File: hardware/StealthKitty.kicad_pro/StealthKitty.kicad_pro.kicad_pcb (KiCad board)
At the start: 4 copper layers, 53.9 x 57 mm, 82 parts, among them IC501 MP1475DJ-LF-P, J201 Conn_01x06, J202 Conn_01x06, J301 Conn_01x06, J302 Conn_01x06, J303 Conn_01x08, J401 Conn_ST_STDC14, SW401 SW_Push, SW402 SW_Push, SW501 Switch, U1 ZXBM5210-SP, U2 ZXBM5210-SP, U301 ADXL343, U401 STM32G431CBU6, Y401 Crystal_GND24_Small

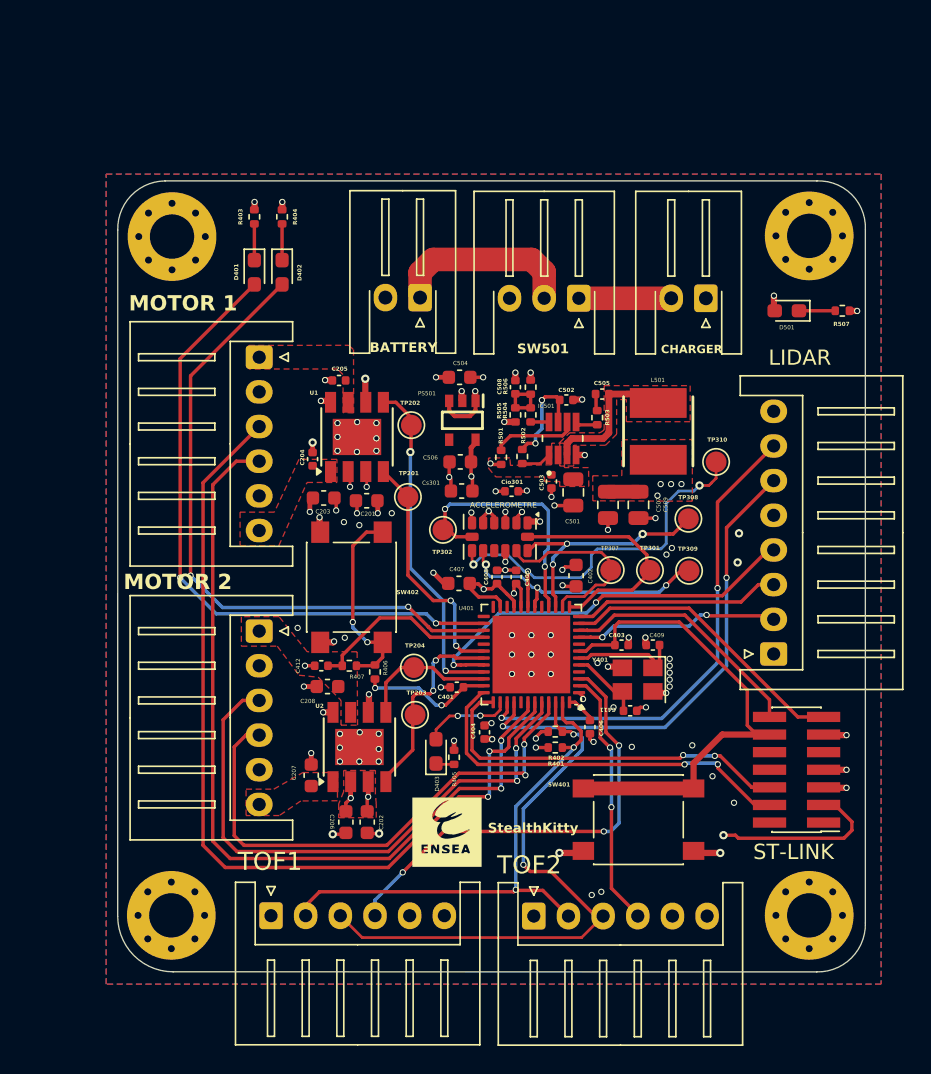
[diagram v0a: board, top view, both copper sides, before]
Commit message: Ajout fichier GERBER zip
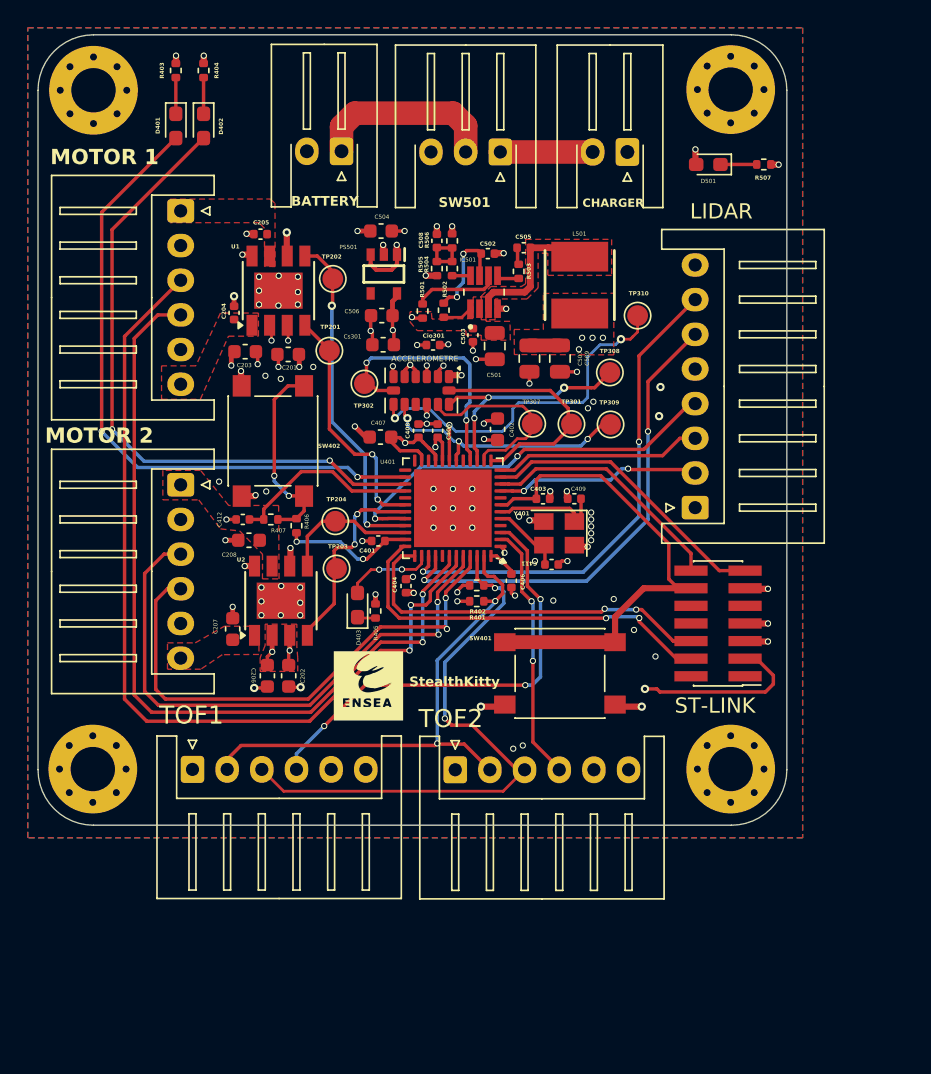
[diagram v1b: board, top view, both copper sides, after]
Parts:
- moved C206 12.0 mm to (135.1, 102.2)
- moved C509 12.0 mm to (154.6, 79.3)
- moved Cs301 12.0 mm to (141.9, 78.3)
- moved J302 12.0 mm to (128.1, 109.0)
- moved J303 12.0 mm to (164.4, 90.1)
- moved R401 12.0 mm to (148.6, 96.8)
- moved BT501 12.0 mm to (138.9, 64.4)
- moved C204 12.0 mm to (131.1, 76.0)
- moved C402 12.0 mm to (150.1, 84.5)
- moved C406 12.0 mm to (151.1, 95.4)
- moved C508 12.0 mm to (145.8, 70.9)
- moved H402 12.0 mm to (166.9, 60.0)
- moved H403 12.0 mm to (166.9, 109.0)
- moved R402 12.0 mm to (148.6, 95.7)
- moved R406 12.0 mm to (135.6, 91.4)
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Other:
- board size 53.9 x 57 mm -> 54 x 57 mm

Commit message: Ajout fichier GERBER final
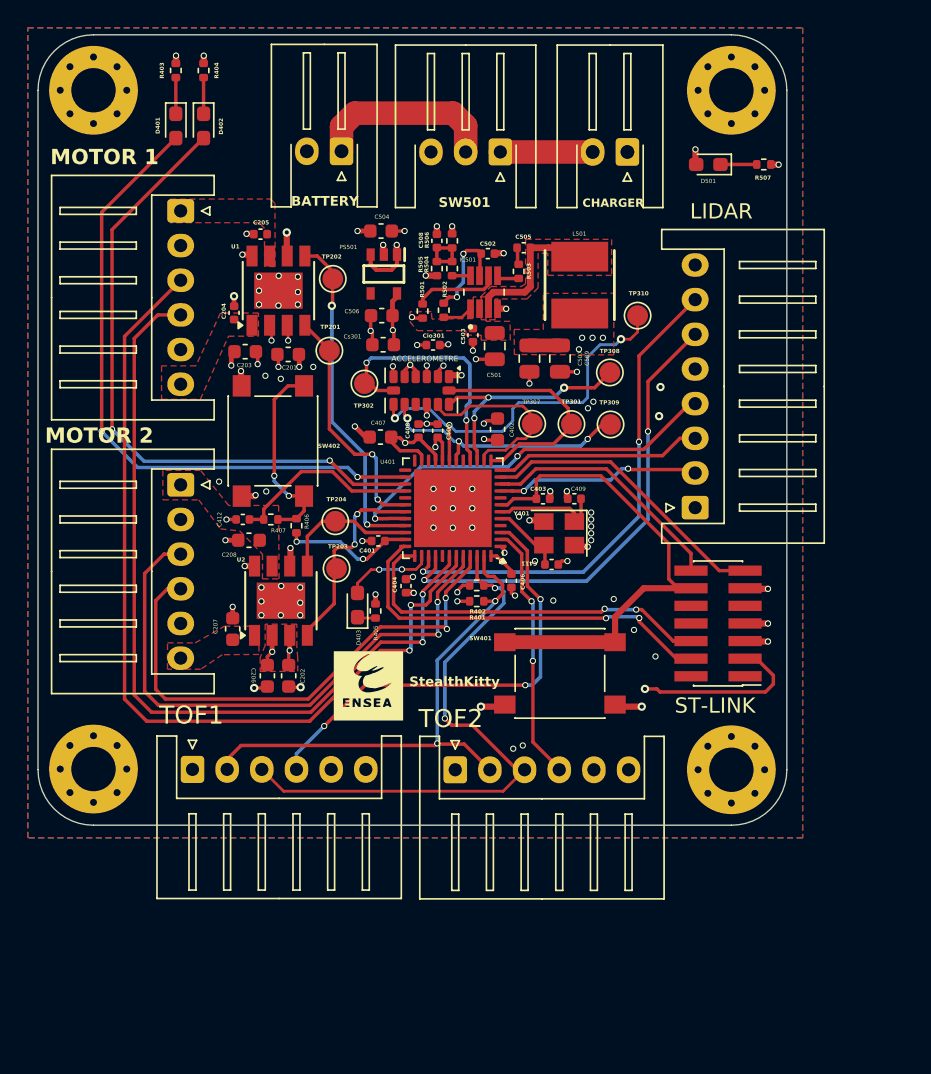
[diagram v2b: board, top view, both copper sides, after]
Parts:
- moved H402 0.07 mm to (167.0, 60.0)
- moved H403 0.07 mm to (167.0, 109.0)
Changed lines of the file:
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@@
 	(footprint "MountingHole:MountingHole_3.2mm_M3_Pad_Via"
 		(layer "F.Cu")
-		(at 166.95 59.95)
+		(at 167 60)
 		(descr "Mounting Hole 3.2mm, M3")
 		(tags "mounting hole 3.2mm m3")
@@
 	(footprint "MountingHole:MountingHole_3.2mm_M3_Pad_Via"
 		(layer "F.Cu")
-		(at 120.95 108.95)
+		(at 121 108.95)
 		(descr "Mounting Hole 3.2mm, M3")
 		(tags "mounting hole 3.2mm m3")
@@
 	(footprint "MountingHole:MountingHole_3.2mm_M3_Pad_Via"
 		(layer "B.Cu")
-		(at 166.95 108.95 180)
+		(at 167 109 180)
 		(descr "Mounting Hole 3.2mm, M3")
 		(tags "mounting hole 3.2mm m3")
